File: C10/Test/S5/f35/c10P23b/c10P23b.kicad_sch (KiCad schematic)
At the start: 5 parts

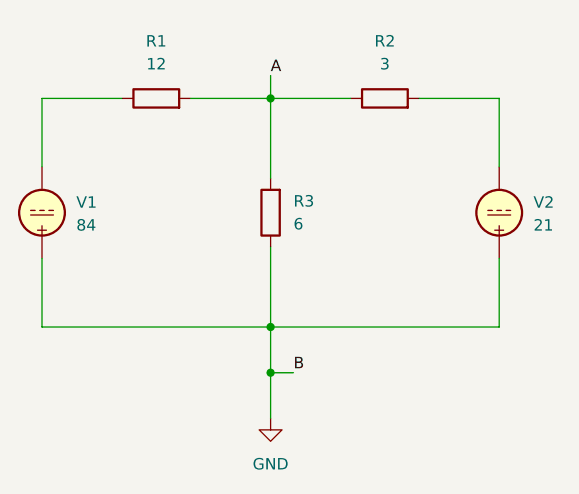
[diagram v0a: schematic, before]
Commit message: additiona upload Chapter 10
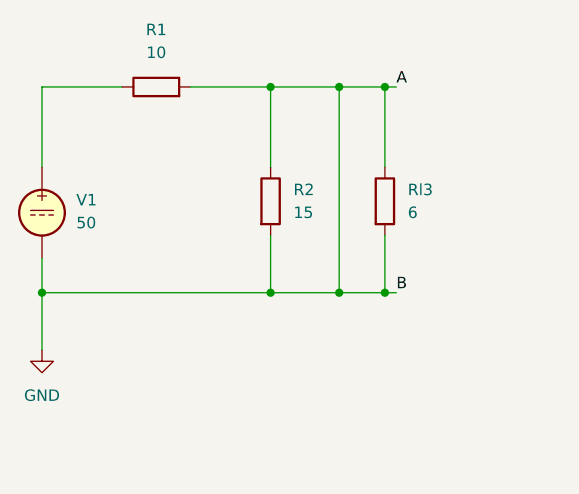
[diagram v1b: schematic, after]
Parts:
- removed R3: 6, symbol Device:R
- removed V2: 21, symbol Simulation_SPICE:VDC
- added Rl3: 6, symbol Device:R
- R1: value 12 -> 10
- R2: value 3 -> 15
- V1: value 84 -> 50
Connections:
- net A is gone; now on net GND: R1.2, R2.1
- net GND: now also R2.2, V1.2, Rl3.1, Rl3.2; no longer V1.1
- net at R1.1: now also V1.1; no longer V1.2
